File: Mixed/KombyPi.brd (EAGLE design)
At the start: 63.2 x 57.1 mm, 16 parts, among them IC3 DS1307, J1 POWER_JACKPTH, J2 MOLEX-39501XXX4, Q1 32.768

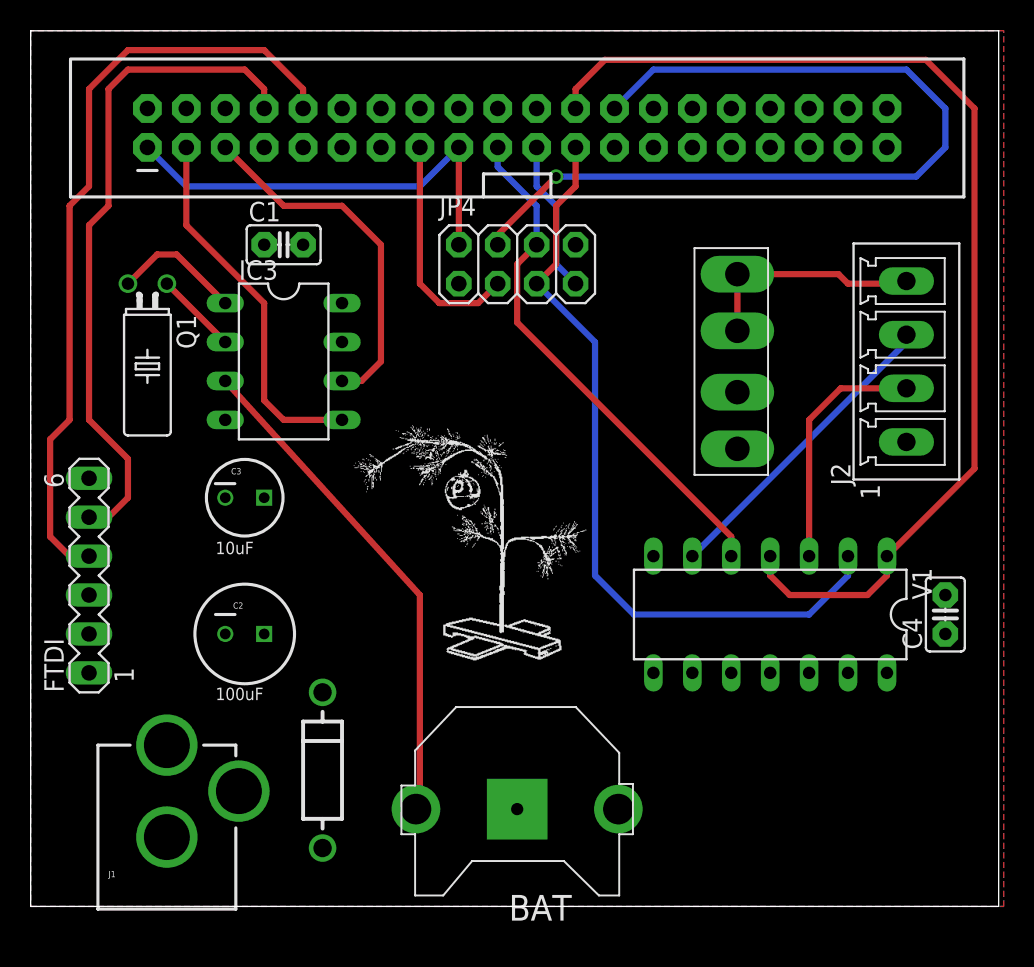
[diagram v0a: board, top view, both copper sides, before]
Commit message: Update KombyPi mixed boards to be cleaner layout.
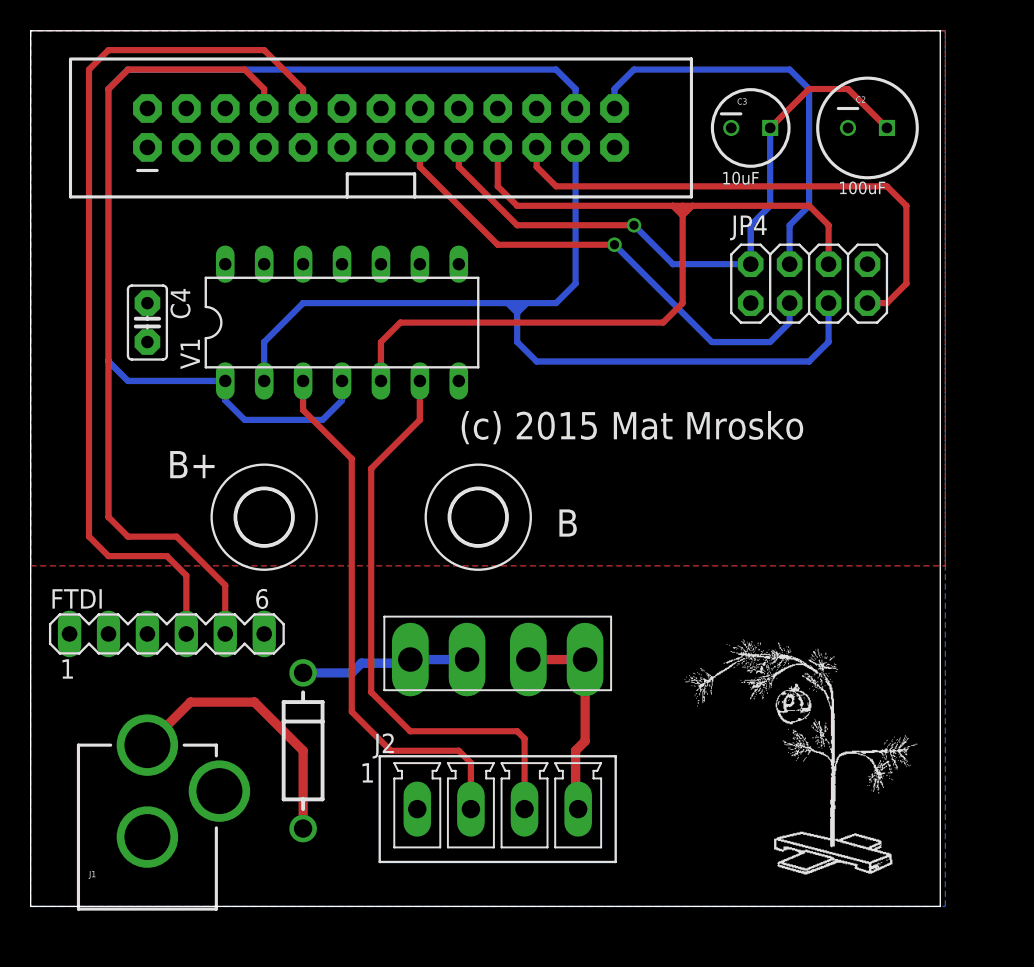
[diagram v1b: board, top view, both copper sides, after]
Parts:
- removed BAT: CR1220, adafruit:CR1220-THM
- removed C1: 0.1uF, adafruit:C025-025X050
- removed IC3: DS1307, adafruit:DIL08
- removed JP3: RASPBERRYPI-B+-GPIO, SparkFun-Boards:2X20-SHROUDED
- removed Q1: 32.768, crystal:TC38H
- added JP1: RASPBERRYPI-GPIOPTH, SparkFun-Boards:2X13-SHROUDED
- added U$2: (no value), holes:3,6
- added U$3: (no value), DIYChristmas-org:DIYC
- U$1: device DIYChristmas-org:DIYC -> holes:3,6
- moved C4 55.4 mm to (7.62, 38.1), turned to 270 degrees
- moved C2 52.4 mm to (54.6, 50.8)
- moved C3 40.9 mm to (47.0, 50.8)
- moved J2 39.6 mm to (30.5, 6.35), turned to 0 degrees
- moved V1 33.8 mm to (20.3, 38.1), turned to 0 degrees
- moved F2 24.4 mm to (30.5, 16.5), turned to 180 degrees
- moved JP4 19.1 mm to (50.8, 40.6)
- moved U$1 13.5 mm to (29.2, 25.4)
- moved FTDI 6.35 mm to (8.89, 17.8), turned to 0 degrees
- moved D1 1.80 mm to (17.8, 5.08)
- moved J1 1.27 mm to (7.62, -3.17)
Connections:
- removed net N$14: IC3.1, Q1.2
- removed net N$15: IC3.2, Q1.1
- removed net N$39: BAT.+2, IC3.3
- removed net SQW: IC3.7
- new net WS2801_VCC_FUSED: F2.P$1, F2.P$2, J2.4
- net 3.3V: now also JP1.1, JP1.17; no longer JP3.1, JP3.17
- net CE0: now also JP1.24; no longer JP3.24
- net CE1: now also JP1.26; no longer JP3.26
- net GND: now also JP1.14, JP1.20, JP1.25, JP1.6, JP1.9; no longer BAT.-, C1.2, IC3.4, JP3.14, JP3.20, JP3.25, JP3.30, JP3.34, JP3.39, JP3.6, JP3.9
- net MISO: now also JP1.21; no longer JP3.21
- net MOSI: now also JP1.19; no longer JP3.19
- net RF_CE: now also JP1.15; no longer JP3.15
- net RXI: now also JP1.10; no longer JP3.10
- net SCL: now also JP1.5; no longer IC3.6, JP3.5
- net SCLK: now also JP1.23; no longer JP3.23
- net SDA: now also JP1.3; no longer IC3.5, JP3.3
- net TXO: now also JP1.8; no longer JP3.8
- net VCC: now also JP1.2, JP1.4; no longer C1.1, D1.C, F2.P$3, F2.P$4, IC3.8, JP3.2, JP3.4
- net WS2801_VCC: now also D1.C, F2.P$3, F2.P$4; no longer F2.P$1, F2.P$2, J2.4
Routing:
- net N$39: track 33.0 -> 0.00 mm
- net CE1: track 58.4 -> 27.0 mm, vias 1 -> 0
- net MOSI: track 34.0 -> 59.1 mm
- net MISO: track 9.94 -> 34.6 mm
- net SDA: track 24.2 -> 0.00 mm
- net SCL: track 23.5 -> 0.00 mm
- net WS2801_SCLK: track 16.1 -> 35.1 mm
- net N$3: track 0.00 -> 17.7 mm
- net WS2801_MOSI: track 20.2 -> 37.5 mm
- net RF_CE: track 15.0 -> 31.9 mm, vias 0 -> 1
- net WS2801_VCC_FUSED: track 0.00 -> 13.8 mm
- net 3.3V: track 29.2 -> 42.1 mm, vias 0 -> 1
- net SCLK: track 50.5 -> 61.6 mm
- net TXO: track 43.8 -> 53.1 mm
- net N$14: track 8.45 -> 0.00 mm
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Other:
- board size 63.2 x 57.1 mm -> 59.4 x 57.1 mm
- board text added: "(c) 2015 Mat Mrosko"
- board text added: "B"
- board text added: "B+"
